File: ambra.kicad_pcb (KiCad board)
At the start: 2 copper layers, 129.8 x 98.6 mm, 33 parts, among them J1 MJ-4PP-9, SW1 SW_SPDT, U1 ProMicro_r

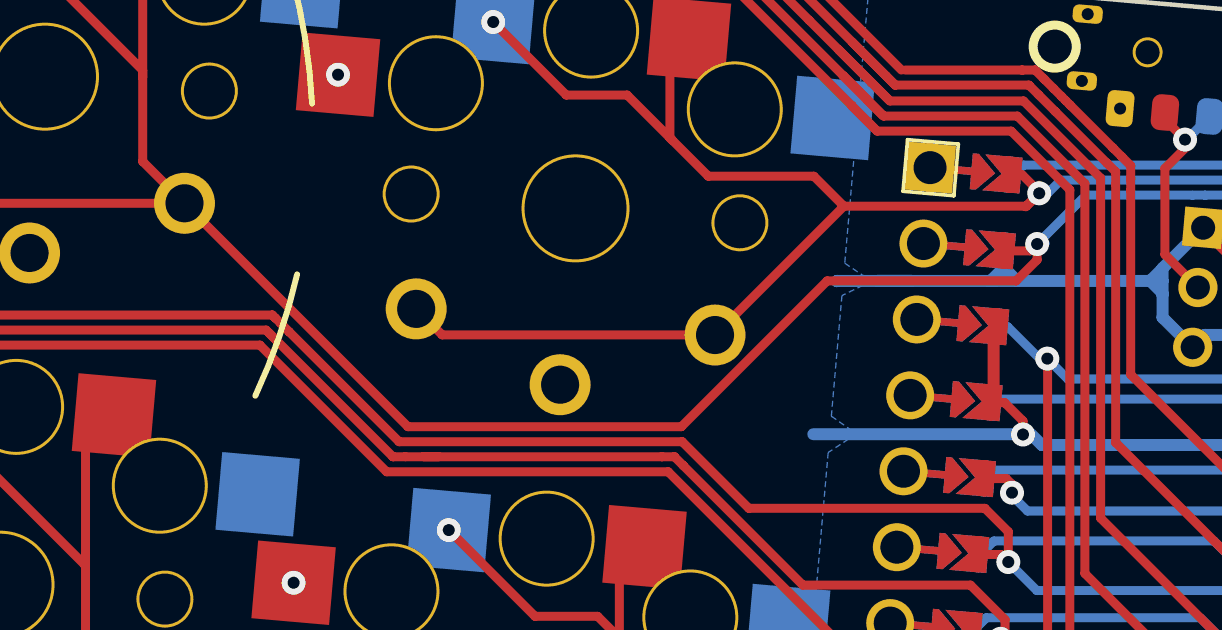
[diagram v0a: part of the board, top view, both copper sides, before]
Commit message: Add files via upload
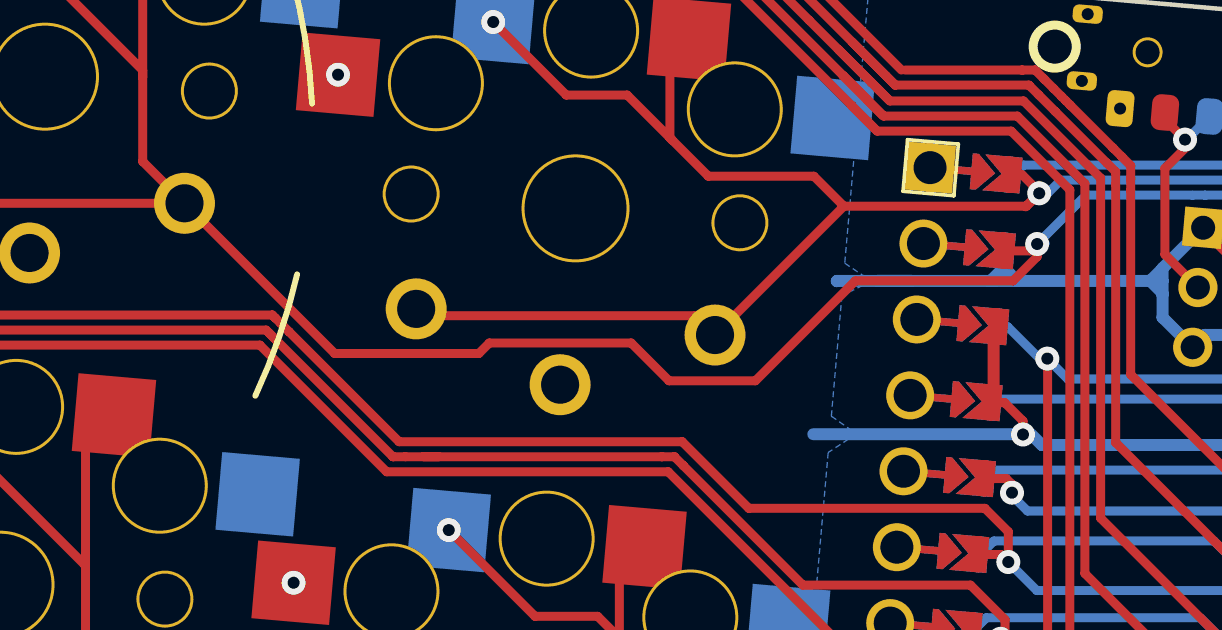
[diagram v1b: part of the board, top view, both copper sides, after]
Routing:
- net r2c2: track 76.8 -> 75.8 mm

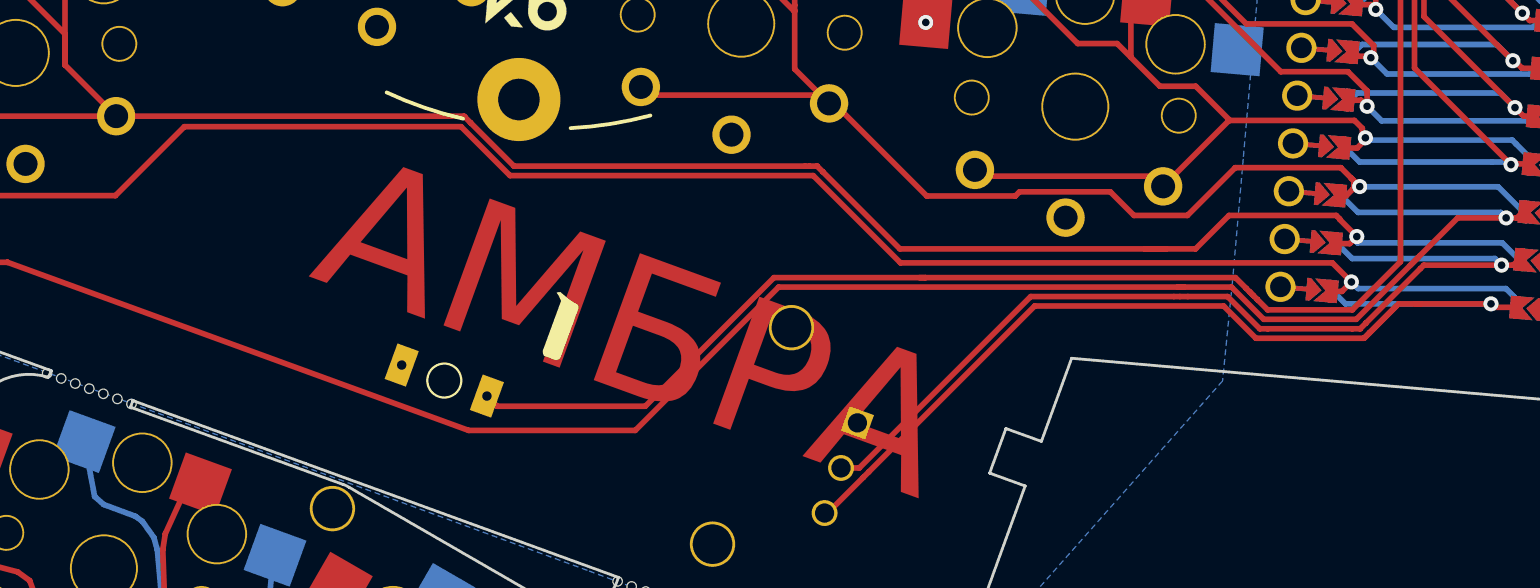
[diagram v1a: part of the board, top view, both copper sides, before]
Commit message: Add files via upload
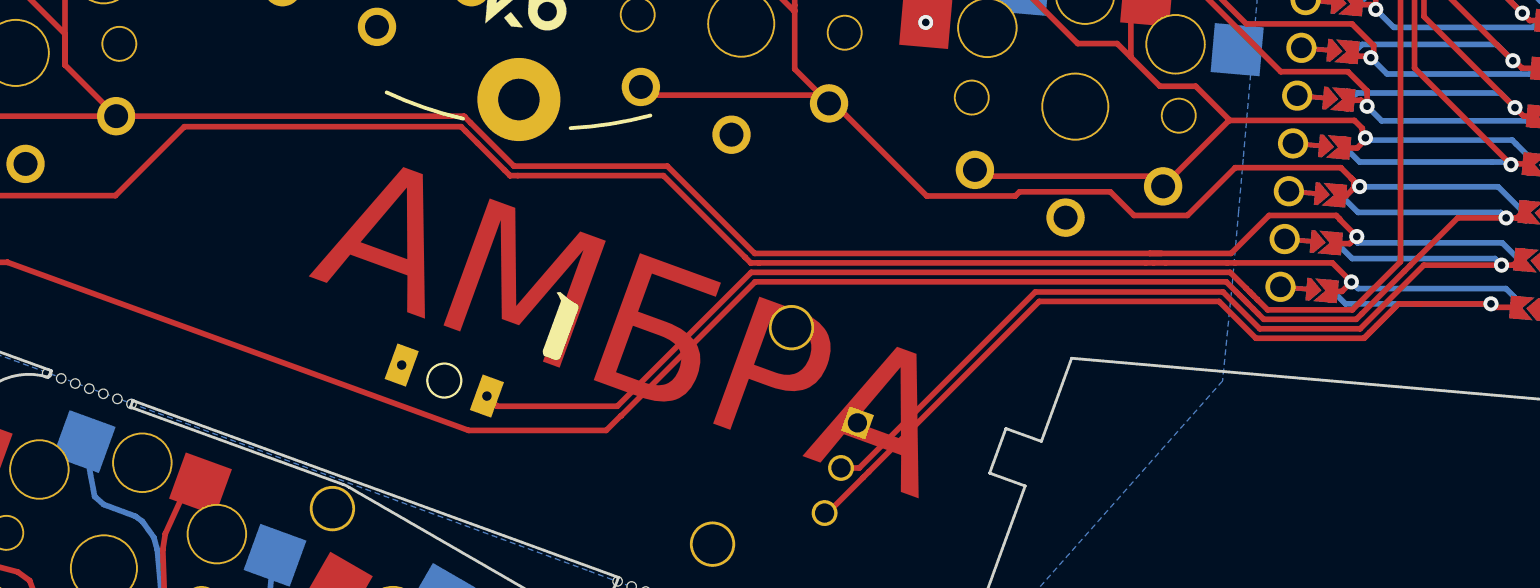
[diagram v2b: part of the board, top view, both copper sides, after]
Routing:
- net r3c5: track 143.9 -> 143.2 mm
